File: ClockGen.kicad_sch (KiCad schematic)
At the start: 37 parts, among them Q10 KT315D, Q11 KT315D, Q5 KT315D, Q6 KT315D, U1 CD4017, U2 CD4017, U3 CD4017, U4 CD4017, U5 CD4017, U6 CD4017, U7 CD4017, Y1 4MHz

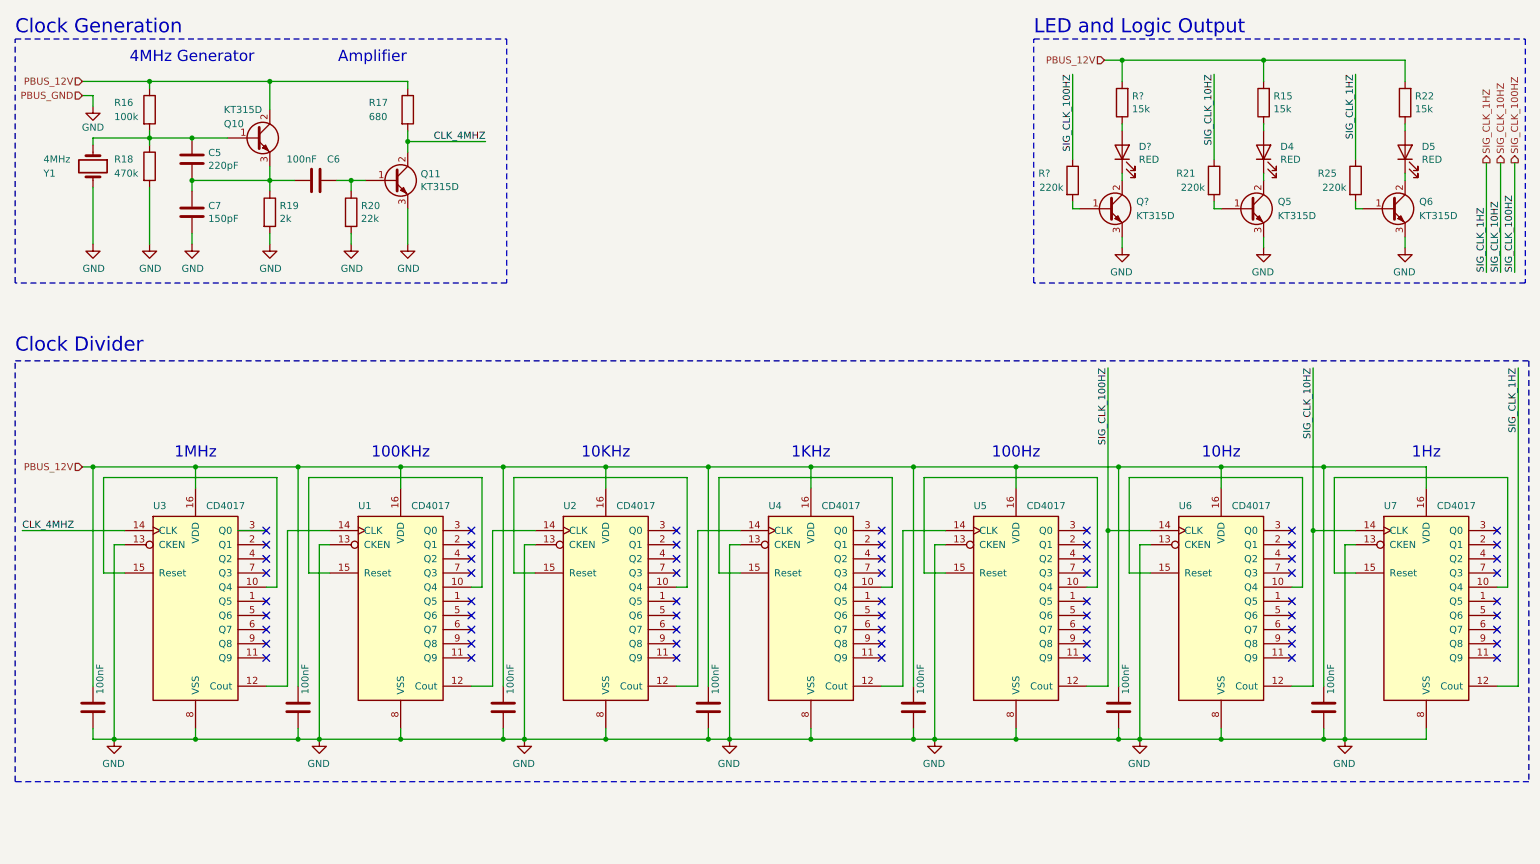
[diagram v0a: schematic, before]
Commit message: Started PCB Outline & PSU
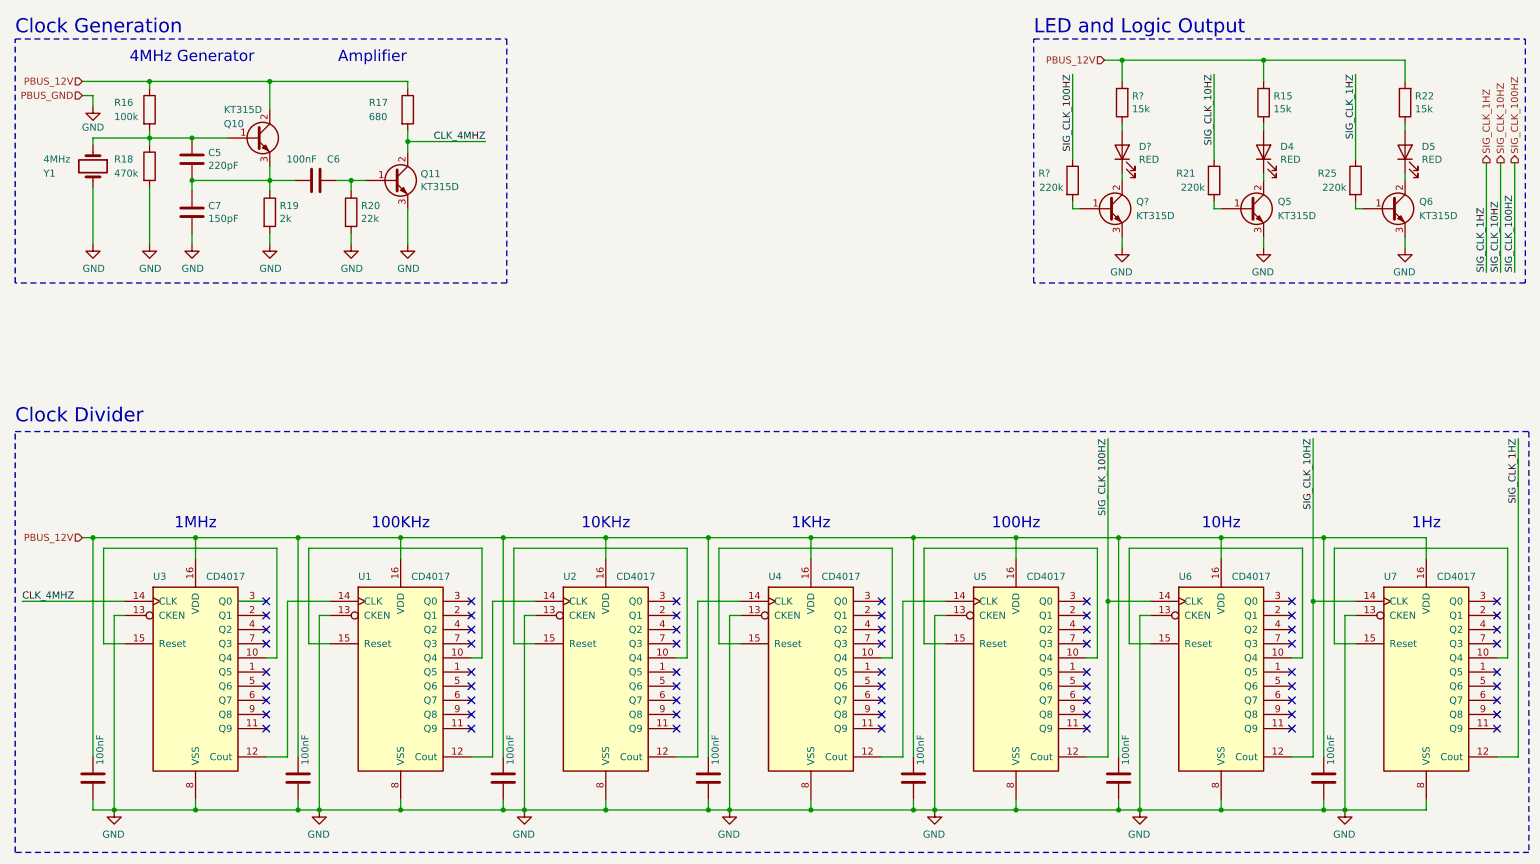
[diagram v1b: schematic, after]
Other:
- moved on the sheet: U1, U2, U3, U4, U5, U6, U7
